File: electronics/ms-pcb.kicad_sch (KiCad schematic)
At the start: 37 parts, among them J1 Left motor, J2 Right motor, J3 XT60-M, U1 ESP32-S3-DEVKITC-1U-N8R2, U2 GY-521

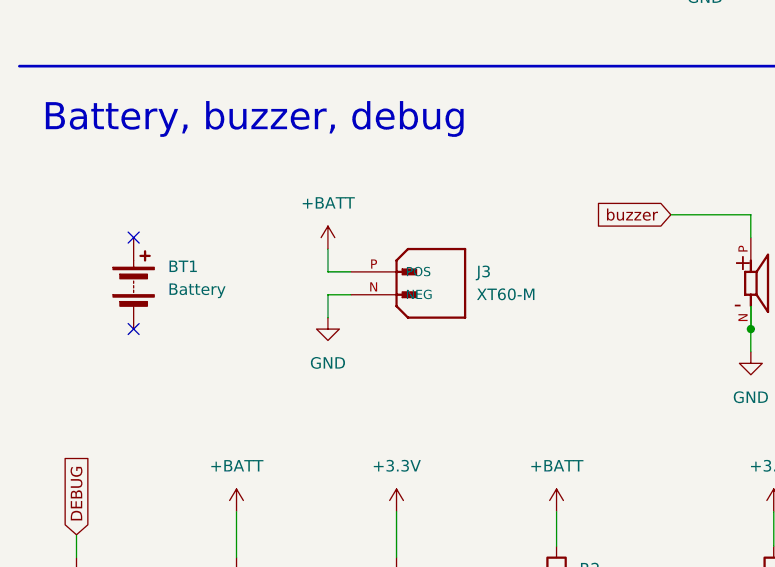
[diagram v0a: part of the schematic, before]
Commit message: elec: final check for PCB v1.1.0
Refs: #51
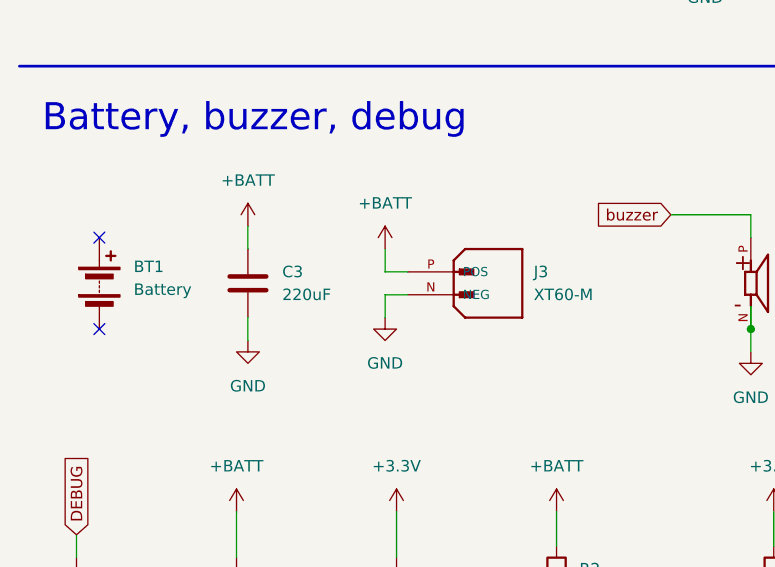
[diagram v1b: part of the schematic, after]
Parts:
- added C3: 220uF, Capacitor_SMD:CP_Elec_8x10.5, symbol Device:C
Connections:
- net +BATT: now also C3.1
- net GND: now also C3.2
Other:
- moved on the sheet: BT1, J3
